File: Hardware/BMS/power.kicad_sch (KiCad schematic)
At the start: 33 parts, among them Q601 SQ2337ES

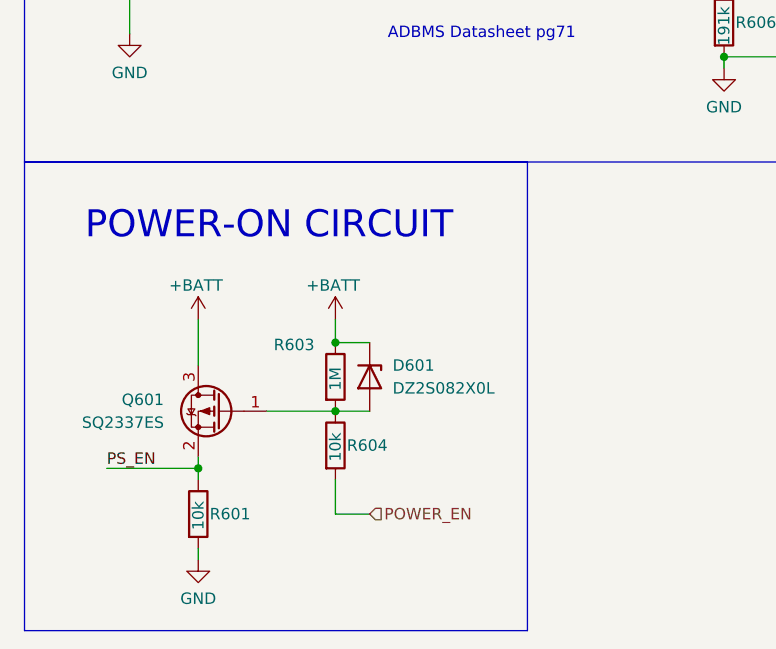
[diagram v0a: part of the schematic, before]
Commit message: bms gotten to 0 unrouted traces!
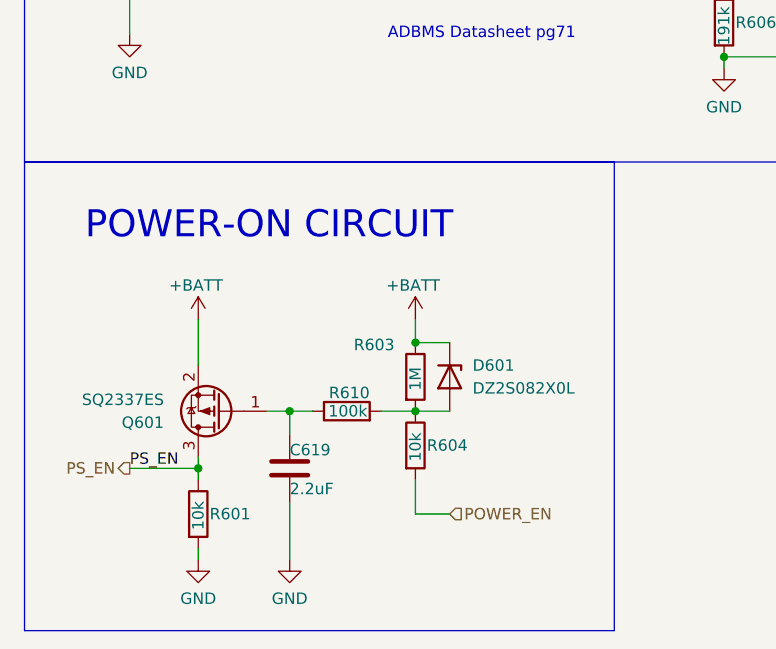
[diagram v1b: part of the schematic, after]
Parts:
- added C619: 2.2uF, Capacitor_SMD:C_0603_1608Metric, symbol Device:C
- added R610: 100k, Resistor_SMD:R_0603_1608Metric, symbol Device:R
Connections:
- net +BATT: now also Q601.2 (S); no longer Q601.3 (D)
- net GND: now also C619.2
- net PS_EN: now also Q601.3 (D); no longer Q601.2 (S)
- net at D601.2 (A), R603.2, R604.1: now also R610.2; no longer Q601.1 (G)
- new net: C619.1, Q601.1 (G), R610.1
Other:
- moved on the sheet: D601, Q601, R603, R604

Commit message: fab updates to bms, power board, fet board
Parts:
- C601, C610, C619: footprint Capacitor_SMD:C_0603_1608Metric -> Capacitor_SMD:C_0805_2012Metric
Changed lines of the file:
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@@
 			)
 		)
-		(property "Footprint" "Capacitor_SMD:C_0603_1608Metric"
+		(property "Footprint" "Capacitor_SMD:C_0805_2012Metric"
 			(at 37.7952 64.77 0)
 			(effects
@@
 			)
 		)
-		(property "Footprint" "Capacitor_SMD:C_0603_1608Metric"
+		(property "Footprint" "Capacitor_SMD:C_0805_2012Metric"
 			(at 55.5752 143.51 0)
 			(effects
@@
 			)
 		)
-		(property "Footprint" "Capacitor_SMD:C_0603_1608Metric"
+		(property "Footprint" "Capacitor_SMD:C_0805_2012Metric"
 			(at 163.5252 64.77 0)
 			(effects
